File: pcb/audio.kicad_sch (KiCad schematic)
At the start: 18 parts, among them U12 CMM4030D, U13 CMM4030D, U14 MAX98357A, U15 MAX98357A

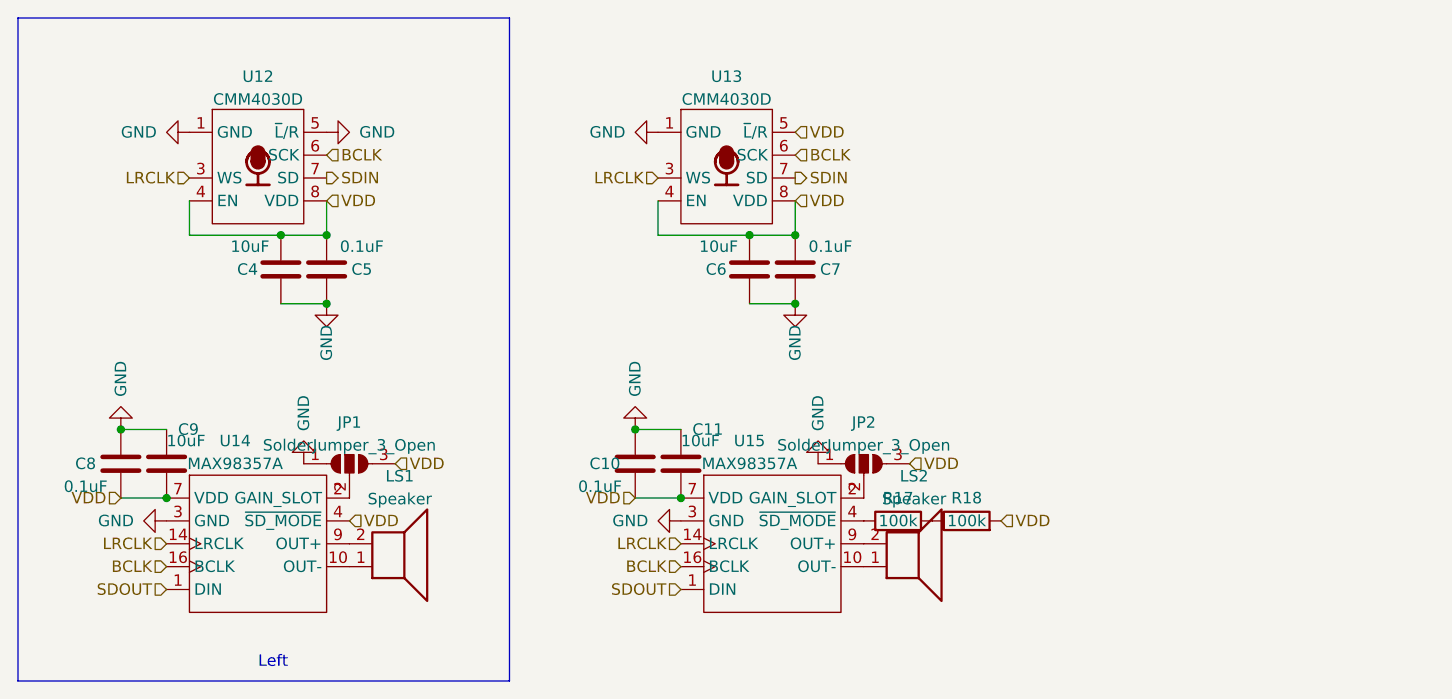
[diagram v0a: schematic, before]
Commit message: v2
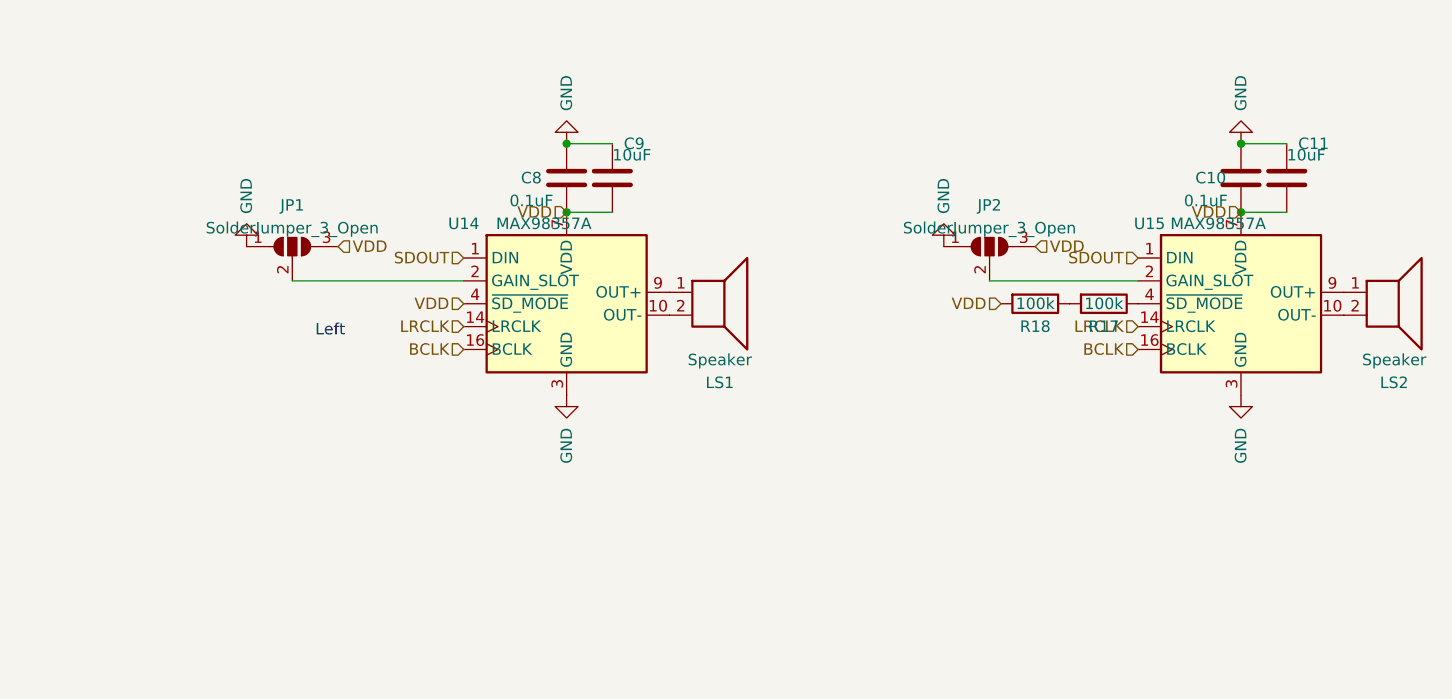
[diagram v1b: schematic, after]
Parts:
- removed C4, C6: 10uF, Capacitor_SMD:C_0603_1608Metric, symbol Device:C
- removed C5, C7: 0.1uF, Capacitor_SMD:C_0603_1608Metric, symbol Device:C
- removed U12, U13: CMM4030D, ic:CMM4030D_hand_solder, symbol ic:CMM4030D
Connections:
- net at LS1.1: now also U14.9 (OUT+); no longer U14.10 (OUT-)
- net at LS1.2: now also U14.10 (OUT-); no longer U14.9 (OUT+)
- net at LS2.1: now also U15.9 (OUT+); no longer U15.10 (OUT-)
- net at LS2.2: now also U15.10 (OUT-); no longer U15.9 (OUT+)
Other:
- moved on the sheet: C10, C11, C8, C9, JP1, JP2, LS1, LS2, R17, R18
